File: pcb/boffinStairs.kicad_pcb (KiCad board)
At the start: 2 copper layers, 17.8 x 19.7 mm, 7 parts, among them P1 CONN_01X05, U1 LM393

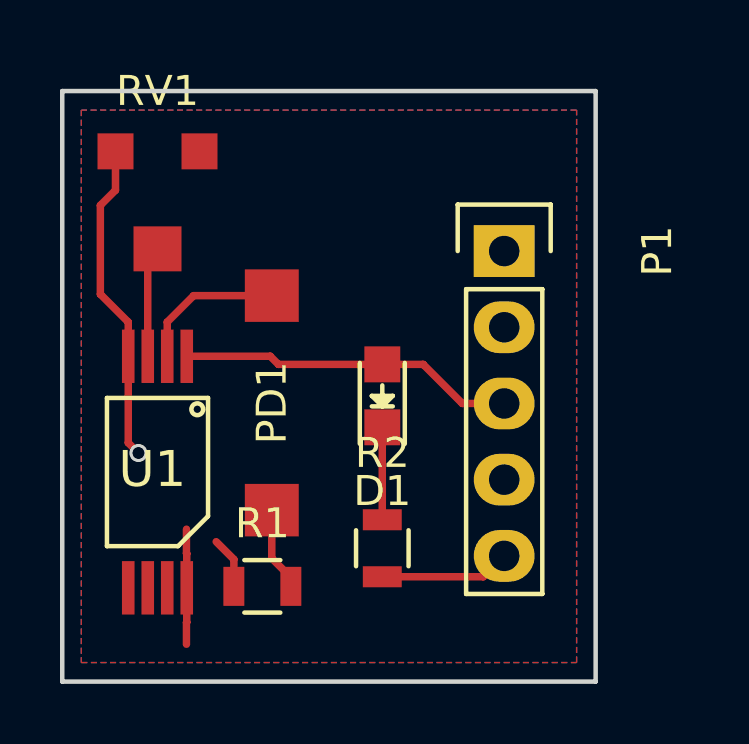
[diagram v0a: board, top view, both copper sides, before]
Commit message: new file:   bf.kicad_mod 	modified:   boffinStairs-B.Cu.gbr 	modified:   boffinStairs-B.Mask.gbr 	modified:   boffinStairs-B.SilkS.gbr 	modified:   boffinStairs-Edge.Cuts.gbr 	modified:   boffinStairs-F.Cu.gbr 	modified:   boffinStairs-F.Mask.gbr 	modified:   boffinStairs-F.SilkS.gbr 	modified:   boffinStairs.drl 	modified:   boffinStairs.kicad_pcb 	modified:   boffinStairs.kicad_pcb-bak 	modified:   fp-lib-table 	new file:   fp.kicad_mod 	deleted:    3361P-104GLFCT-ND.pretty/3361P Bourns trimming Potentiometer.kicad_mod 	deleted:    pianostairs-cache.lib 	deleted:    pianostairs.bak 	deleted:    pianostairs.kicad_pcb 	deleted:    pianostairs.kicad_pcb-bak 	deleted:    pianostairs.net 	deleted:    pianostairs.pro 	deleted:    pianostairs.sch 	deleted:    pianostairs.xml
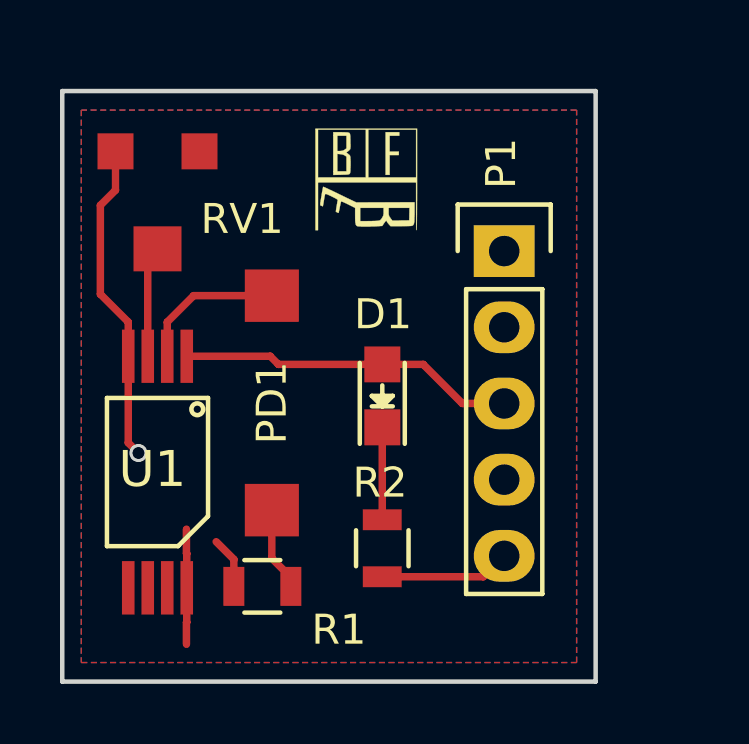
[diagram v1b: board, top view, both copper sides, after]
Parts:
- added G***: LOGO, boffinStairs:bf, F.Cu at (160.0, 100.7)
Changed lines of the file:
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@@
 (kicad_pcb (version 4) (host pcbnew 0.201511192131+6326~38~ubuntu14.04.1-stable)
   (general
-    (links 14)
+    (links 0)
     (no_connects 0)
-    (area 149.01156 96.665 170.667 117.550001)
+    (area 149.01156 97.714999 168.667 117.550001)
     (thickness 1.6)
     (drawings 4)
     (tracks 34)
     (zones 0)
-    (modules 7)
+    (modules 8)
     (nets 8)
   )
@@
     (tags "LED 0805 SMD")
     (attr smd)
-    (fp_text reference D1 (at -3.175 0 180) (layer F.SilkS)
+    (fp_text reference D1 (at 2.7178 0.0254 180) (layer F.SilkS)
       (effects (font (size 1 1) (thickness 0.15)))
     )
@@
     (tags "resistor 0805")
     (attr smd)
-    (fp_text reference R1 (at 0 -2.1) (layer F.SilkS)
+    (fp_text reference R1 (at 2.5502 1.4478) (layer F.SilkS)
       (effects (font (size 1 1) (thickness 0.15)))
     )
@@
     (tags "resistor 0805")
     (attr smd)
-    (fp_text reference R2 (at -3.175 0 360) (layer F.SilkS)
+    (fp_text reference R2 (at -2.1844 0.0762 360) (layer F.SilkS)
       (effects (font (size 1 1) (thickness 0.15)))
     )
@@
   (module PD70:TC33 (layer F.Cu)
     (at 153.035 101.6 180)
-    (fp_text reference RV1 (at 0 3.81 180) (layer F.SilkS)
+    (fp_text reference RV1 (at -2.8194 -0.4572 180) (layer F.SilkS)
       (effects (font (size 1 1) (thickness 0.15)))
     )
@@
     (descr "Through hole socket strip")
     (tags "socket strip")
-    (fp_text reference P1 (at 0 -5.1 270) (layer F.SilkS)
+    (fp_text reference P1 (at -2.921 0.1016 270) (layer F.SilkS)
       (effects (font (size 1 1) (thickness 0.15)))
     )
@@
     )
   )
+  (module boffinStairs:bf (layer F.Cu)
+    (at 159.9946 100.7364)
+    (fp_text reference G*** (at 0 0) (layer F.SilkS) hide
+      (effects (font (thickness 0.3)))
+    )
+    (fp_text value LOGO (at 0.75 0) (layer F.SilkS) hide
+      (effects (font (thickness 0.3)))
+    )
+    (fp_poly (pts (xy 1.693333 0) (xy 1.693164 0.316) (xy 1.692658 0.599929) (xy 1.691818 0.851591)
+      (xy 1.690645 1.070788) (xy 1.689141 1.257324) (xy 1.687308 1.410999) (xy 1.685149 1.531619)
+      (xy 1.682665 1.618984) (xy 1.679857 1.672899) (xy 1.676729 1.693165) (xy 1.6764 1.693333)
+      (xy 1.671983 1.676501) (xy 1.668212 1.626401) (xy 1.665097 1.543625) (xy 1.662653 1.428765)
+      (xy 1.660891 1.282412) (xy 1.659825 1.105161) (xy 1.659467 0.897602) (xy 1.659466 0.897467)
+      (xy 1.659466 0.1016) (xy -1.608667 0.1016) (xy -1.608667 1.693333) (xy -1.693333 1.693333)
+      (xy -1.693333 -1.659467) (xy -1.608667 -1.659467) (xy -1.608667 -0.067733) (xy -0.016934 -0.067733)
+      (xy -0.016934 -1.659467) (xy 0.067733 -1.659467) (xy 0.067733 -0.067733) (xy 1.659466 -0.067733)
+      (xy 1.659466 -1.659467) (xy 0.067733 -1.659467) (xy -0.016934 -1.659467) (xy -1.608667 -1.659467)
+      (xy -1.693333 -1.659467) (xy -1.693333 -1.693333) (xy 1.693333 -1.693333) (xy 1.693333 0)) (layer F.SilkS) (width 0.01))
+    (fp_poly (pts (xy -1.419438 0.250202) (xy -1.376025 0.268241) (xy -1.31003 0.297744) (xy -1.225338 0.336932)
+      (xy -1.125836 0.384026) (xy -1.01541 0.43725) (xy -0.988798 0.450209) (xy -0.869852 0.508137)
+      (xy -0.755149 0.563806) (xy -0.64986 0.614719) (xy -0.559155 0.658382) (xy -0.488206 0.6923)
+      (xy -0.442184 0.713979) (xy -0.440267 0.714864) (xy -0.3302 0.765595) (xy 0.639233 0.762718)
+      (xy 1.608666 0.759842) (xy 1.608666 1.100428) (xy 1.607906 1.233116) (xy 1.605096 1.335972)
+      (xy 1.599444 1.41301) (xy 1.590157 1.468242) (xy 1.576443 1.505679) (xy 1.557508 1.529336)
+      (xy 1.532561 1.543223) (xy 1.520445 1.547016) (xy 1.491978 1.550234) (xy 1.435543 1.55307)
+      (xy 1.357038 1.555358) (xy 1.26236 1.55693) (xy 1.157408 1.55762) (xy 1.145284 1.557635)
+      (xy 0.808901 1.557867) (xy 0.751723 1.495443) (xy 0.716087 1.452644) (xy 0.690758 1.415114)
+      (xy 0.684798 1.402309) (xy 0.674192 1.379382) (xy 0.660035 1.376838) (xy 0.638131 1.397347)
+      (xy 0.604287 1.443576) (xy 0.592355 1.461113) (xy 0.532778 1.5494) (xy 0.380689 1.560307)
+      (xy 0.306432 1.564413) (xy 0.216321 1.567527) (xy 0.117205 1.569622) (xy 0.015935 1.570673)
+      (xy -0.080639 1.570653) (xy -0.165669 1.569536) (xy -0.232304 1.567294) (xy -0.273695 1.563903)
+      (xy -0.2794 1.562848) (xy -0.311771 1.551575) (xy -0.335702 1.532194) (xy -0.352433 1.500063)
+      (xy -0.3632 1.450538) (xy -0.369241 1.378979) (xy -0.371793 1.280742) (xy -0.372157 1.214887)
+      (xy -0.372532 0.948267) (xy -0.2032 0.948267) (xy -0.2032 1.388533) (xy 0.031383 1.388533)
+      (xy 0.127626 1.38775) (xy 0.221457 1.385609) (xy 0.302775 1.382429) (xy 0.361482 1.378524)
+      (xy 0.36629 1.378047) (xy 0.423457 1.370608) (xy 0.459517 1.358266) (xy 0.487122 1.333429)
+      (xy 0.518925 1.288506) (xy 0.521174 1.285111) (xy 0.549952 1.238118) (xy 0.566385 1.197529)
+      (xy 0.57385 1.150367) (xy 0.575723 1.083657) (xy 0.575733 1.075463) (xy 0.575733 0.948267)
+      (xy 0.745067 0.948267) (xy 0.745067 1.075227) (xy 0.746308 1.142956) (xy 0.752484 1.189594)
+      (xy 0.767271 1.227893) (xy 0.794347 1.270607) (xy 0.80621 1.287295) (xy 0.867353 1.372402)
+      (xy 1.14911 1.367767) (xy 1.430867 1.363133) (xy 1.435621 1.1557) (xy 1.440376 0.948267)
+      (xy 0.745067 0.948267) (xy 0.575733 0.948267) (xy -0.2032 0.948267) (xy -0.372532 0.948267)
+      (xy -0.372533 0.948107) (xy -0.600386 0.83455) (xy -0.680338 0.795609) (xy -0.749329 0.763722)
+      (xy -0.801874 0.741288) (xy -0.832489 0.730709) (xy -0.837848 0.730604) (xy -0.844698 0.750199)
+      (xy -0.855897 0.795945) (xy -0.869795 0.860662) (xy -0.882397 0.924674) (xy -0.896837 0.999173)
+      (xy -0.909284 1.060177) (xy -0.918284 1.100748) (xy -0.922146 1.114) (xy -0.939567 1.111795)
+      (xy -0.970822 1.098721) (xy -1.001117 1.082002) (xy -1.015657 1.068862) (xy -1.015705 1.068315)
+      (xy -1.01284 1.045966) (xy -1.005657 0.999202) (xy -0.995638 0.936972) (xy -0.984265 0.868227)
+      (xy -0.973021 0.801918) (xy -0.963386 0.746994) (xy -0.956845 0.712408) (xy -0.956519 0.710877)
+      (xy -0.954692 0.692742) (xy -0.960987 0.676525) (xy -0.979952 0.658879) (xy -1.016136 0.636452)
+      (xy -1.074088 0.605896) (xy -1.15172 0.567141) (xy -1.240767 0.524296) (xy -1.303794 0.496973)
+      (xy -1.344202 0.483925) (xy -1.365392 0.483903) (xy -1.369267 0.487291) (xy -1.376984 0.511744)
+      (xy -1.38804 0.562132) (xy -1.400904 0.630879) (xy -1.412886 0.702993) (xy -1.425294 0.779214)
+      (xy -1.436284 0.841414) (xy -1.444633 0.883015) (xy -1.449029 0.897467) (xy -1.466763 0.89123)
+      (xy -1.499619 0.876988) (xy -1.514939 0.870704) (xy -1.526322 0.864702) (xy -1.533602 0.854704)
+      (xy -1.536612 0.836429) (xy -1.535187 0.8056) (xy -1.52916 0.757935) (xy -1.518365 0.689157)
+      (xy -1.502636 0.594985) (xy -1.484478 0.487095) (xy -1.469749 0.402292) (xy -1.456211 0.329982)
+      (xy -1.445121 0.276485) (xy -1.437737 0.248121) (xy -1.436382 0.245404) (xy -1.419438 0.250202)) (layer F.SilkS) (width 0.01))
+    (fp_poly (pts (xy -0.742991 -1.573914) (xy -0.665277 -1.570994) (xy -0.612132 -1.56565) (xy -0.578928 -1.557488)
+      (xy -0.56627 -1.550801) (xy -0.553454 -1.53849) (xy -0.54421 -1.519588) (xy -0.537784 -1.488606)
+      (xy -0.533423 -1.440056) (xy -0.530372 -1.368449) (xy -0.527954 -1.271844) (xy -0.526053 -1.173808)
+      (xy -0.525682 -1.103807) (xy -0.527532 -1.056017) (xy -0.532296 -1.024618) (xy -0.540663 -1.003786)
+      (xy -0.553327 -0.9877) (xy -0.562816 -0.978344) (xy -0.602142 -0.943926) (xy -0.635996 -0.918633)
+      (xy -0.659065 -0.901284) (xy -0.65349 -0.888161) (xy -0.635996 -0.8763) (xy -0.599357 -0.848804)
+      (xy -0.564029 -0.817803) (xy -0.549519 -0.802495) (xy -0.539128 -0.784974) (xy -0.53217 -0.759721)
+      (xy -0.527958 -0.721219) (xy -0.525807 -0.663952) (xy -0.525029 -0.582402) (xy -0.524933 -0.50354)
+      (xy -0.52567 -0.391848) (xy -0.528112 -0.309494) (xy -0.532609 -0.251975) (xy -0.539508 -0.214787)
+      (xy -0.548933 -0.193737) (xy -0.561002 -0.181119) (xy -0.579494 -0.171966) (xy -0.609791 -0.165562)
+      (xy -0.657275 -0.16119) (xy -0.727326 -0.158135) (xy -0.825327 -0.15568) (xy -0.8368 -0.155442)
+      (xy -1.100667 -0.150016) (xy -1.100667 -0.270933) (xy -0.9652 -0.270933) (xy -0.6604 -0.270933)
+      (xy -0.6604 -0.759694) (xy -0.714326 -0.798093) (xy -0.784459 -0.830284) (xy -0.866726 -0.843614)
+      (xy -0.9652 -0.850737) (xy -0.9652 -0.270933) (xy -1.100667 -0.270933) (xy -1.100667 -1.456267)
+      (xy -0.9652 -1.456267) (xy -0.9652 -0.948267) (xy -0.875998 -0.948267) (xy -0.804338 -0.954564)
+      (xy -0.746574 -0.97687) (xy -0.723598 -0.991211) (xy -0.6604 -1.034154) (xy -0.6604 -1.456267)
+      (xy -0.9652 -1.456267) (xy -1.100667 -1.456267) (xy -1.100667 -1.5748) (xy -0.849903 -1.5748)
+      (xy -0.742991 -1.573914)) (layer F.SilkS) (width 0.01))
+    (fp_poly (pts (xy 1.100667 -1.456267) (xy 0.778933 -1.456267) (xy 0.778933 -0.931333) (xy 1.083733 -0.931333)
+      (xy 1.083733 -0.8128) (xy 0.778933 -0.8128) (xy 0.778933 -0.1524) (xy 0.643467 -0.1524)
+      (xy 0.643467 -1.5748) (xy 1.100667 -1.5748) (xy 1.100667 -1.456267)) (layer F.SilkS) (width 0.01))
+  )
   (gr_line (start 149.86 97.79) (end 149.86 117.475) (layer Edge.Cuts) (width 0.15))
